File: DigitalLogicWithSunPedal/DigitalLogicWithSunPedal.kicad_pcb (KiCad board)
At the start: 2 copper layers, 155 x 110 mm, 19 parts, among them IC1 REG1117-5, IC2 HEF4081BT,653, J1 776280-1, J2 4pin brake, J3 4pin throttle, K1 J107F1AS123VDC.36, Q1 2N2222A, U2 TS881ICT, U3 TS881ICT, U4 TS881ICT, U5 TS881ICT

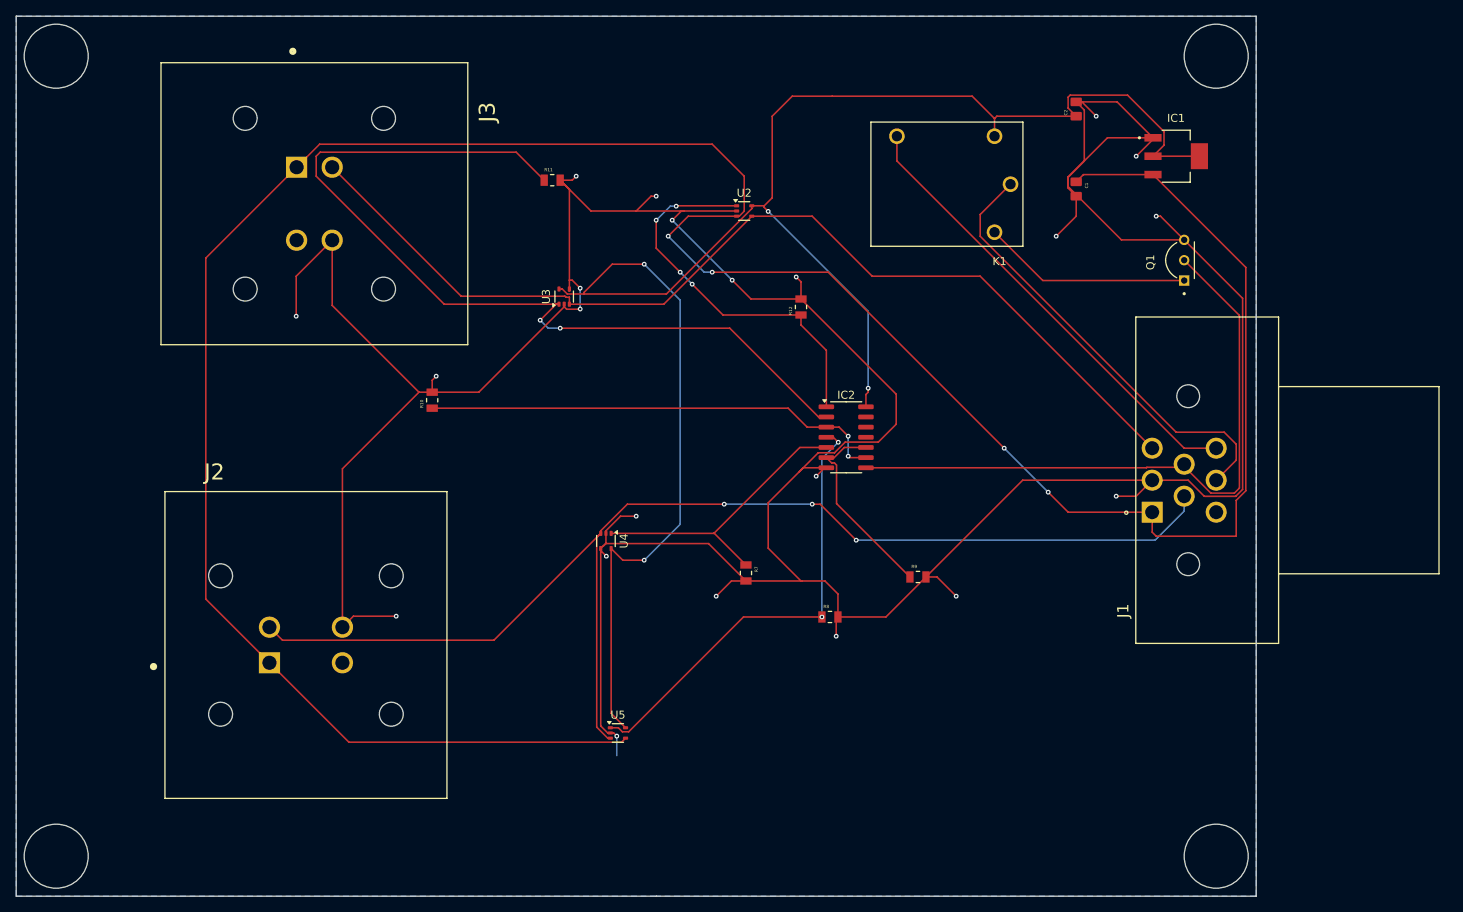
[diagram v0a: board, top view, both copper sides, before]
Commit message: Add files via upload
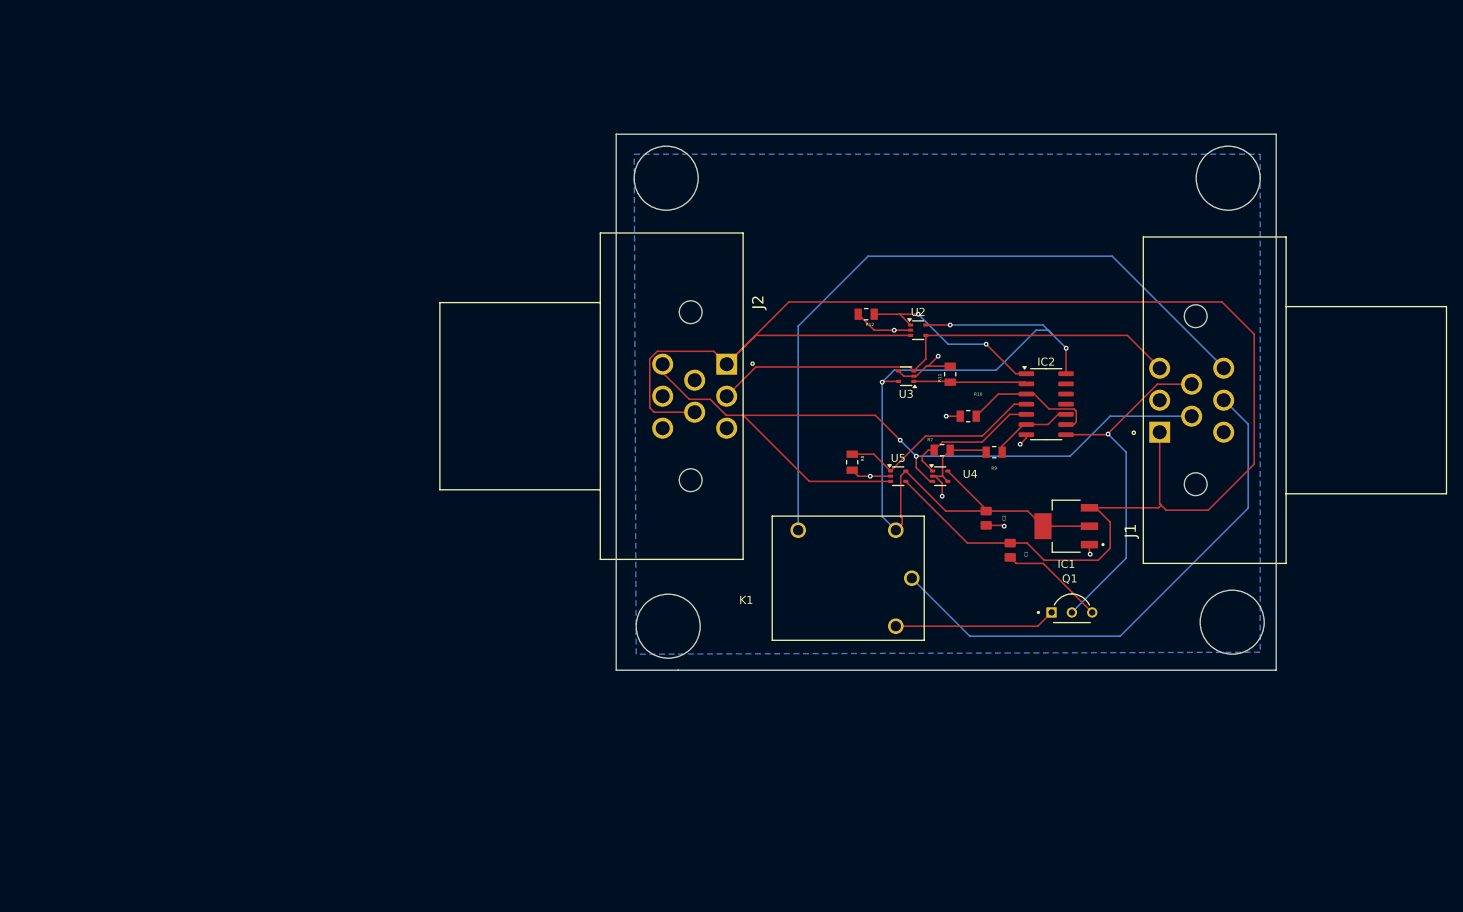
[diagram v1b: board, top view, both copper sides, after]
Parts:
- removed J3: 4pin throttle, DT15-4P:TE_DT15-4P
- J2: value 4pin brake -> 776280-1; footprint DT15-4P:TE_DT15-4P -> 776280-1:TE_776280-1
- moved R10 67.0 mm to (156.5, 82.5), turned to 180 degrees
- moved J2 57.7 mm to (122.3, 80.0), turned to -90 degrees
- moved R11 55.3 mm to (154.2, 77.2), turned to 90 degrees
- moved C2 52.4 mm to (158.8, 95.2), turned to -90 degrees
- moved K1 50.8 mm to (141.5, 102.8)
- moved IC1 48.3 mm to (168.8, 96.2), turned to 180 degrees
- moved U5 47.5 mm to (147.8, 90.0)
- moved C1 45.9 mm to (161.8, 99.2)
- moved U3 43.9 mm to (148.8, 77.5), turned to 180 degrees
- moved Q1 43.3 mm to (169.5, 104.7), turned to 0 degrees
- moved U4 42.6 mm to (153.0, 90.0), turned to 0 degrees
- moved R7 28.9 mm to (153.2, 86.8), turned to 0 degrees
- moved U2 26.4 mm to (150.2, 71.8)
- moved IC2 25.3 mm to (166.2, 81.0)
- moved R8 19.5 mm to (142.0, 88.2), turned to -90 degrees
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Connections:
- J2 pad 2: Net-(U4-+) -> Net-(U2--)
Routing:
- net GND: track 487.6 -> 55.2 mm, vias 22 -> 8
- net +12V: track 341.2 -> 203.6 mm, vias 4 -> 0
- net +5V: track 219.5 -> 108.3 mm, vias 4 -> 3
- net Net-(IC2-Pad2): track 113.6 -> 14.2 mm, vias 2 -> 0
- net Net-(U2--): track 126.7 -> 61.2 mm
- net Net-(U4-+): track 154.2 -> 99.6 mm, vias 3 -> 2
- net Net-(IC2-Pad3): track 58.2 -> 17.3 mm, vias 2 -> 0
- net Net-(IC2-Pad8): track 80.1 -> 44.4 mm, vias 0 -> 1
- net Net-(IC2-Pad4): track 57.0 -> 26.1 mm, vias 2 -> 0
- net Net-(J1-Pad8): track 57.9 -> 88.2 mm
- net Net-(IC2-Pad1): track 48.6 -> 24.0 mm, vias 4 -> 2
- net Net-(IC2-Pad5): track 37.0 -> 17.6 mm
- net Net-(IC2-Pad10): track 24.9 -> 10.4 mm
- net Net-(J1-Pad7): track 56.4 -> 66.4 mm
- net Net-(K1-PadCOIL1): track 26.2 -> 20.2 mm
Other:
- board size 155 x 110 mm -> 82.5 x 67 mm
